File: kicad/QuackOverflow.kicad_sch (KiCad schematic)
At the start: 13 parts, among them J1 Qi_Reciever, U1 ESP32-C3-MINI-1, U2 TP4056-42-ESOP8

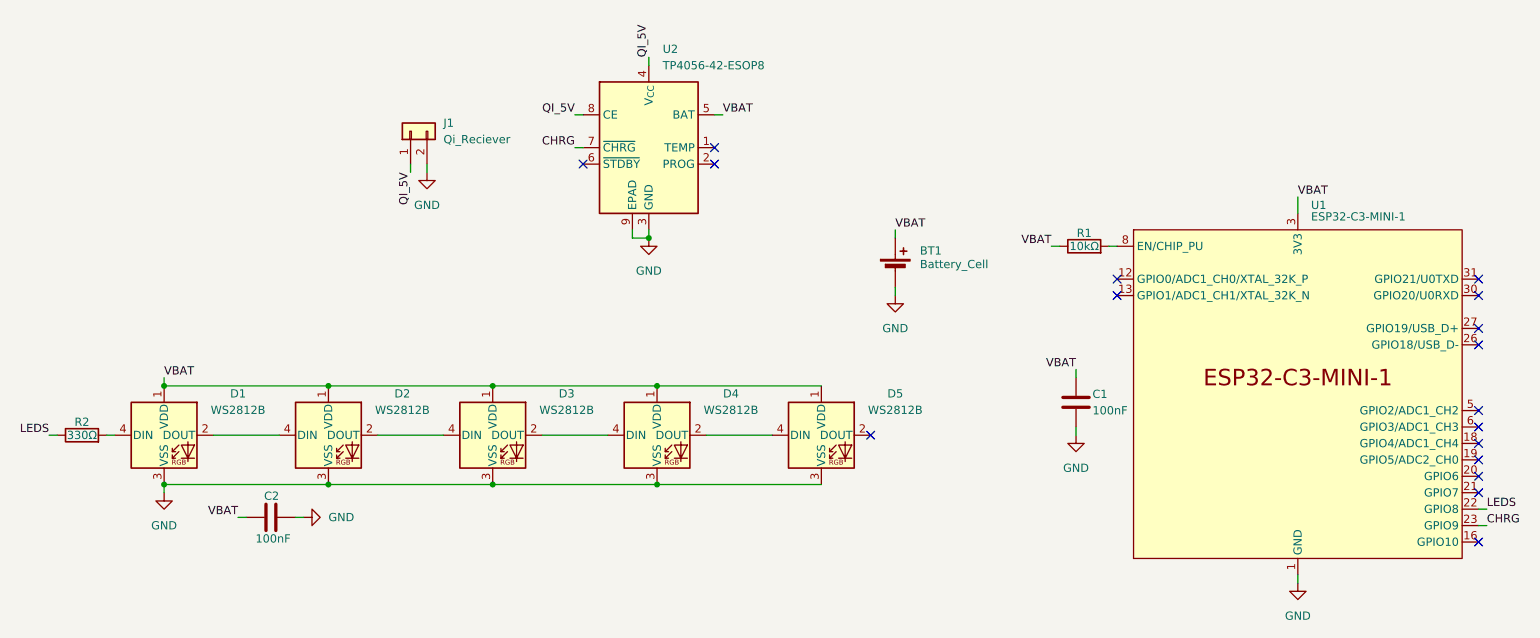
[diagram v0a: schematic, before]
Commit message: PCB\!\!\!
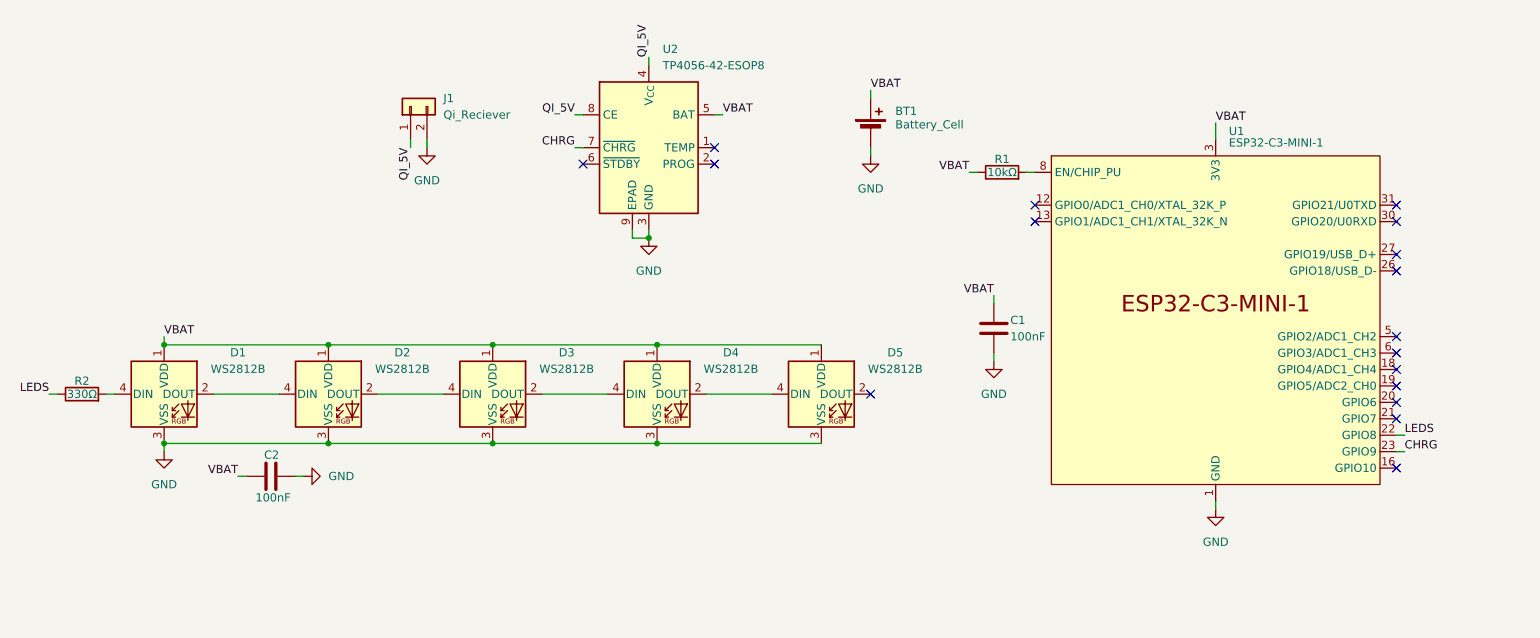
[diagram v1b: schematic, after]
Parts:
- BT1, J1: footprint (none) -> Connector_PinHeader_1.00mm:PinHeader_1x02_P1.00mm_Vertical
- C1, C2: footprint (none) -> Capacitor_SMD:C_1206_3216Metric_Pad1.33x1.80mm_HandSolder
- R1, R2: footprint (none) -> Resistor_SMD:R_1206_3216Metric_Pad1.30x1.75mm_HandSolder
- U1: footprint PCM_Espressif:ESP32-C3-MINI-1 -> Espressif:ESP32-C3-MINI-1
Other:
- moved on the sheet: BT1, C1, C2, D1, D2, D3, D4, D5, J1, R1, R2, U1
